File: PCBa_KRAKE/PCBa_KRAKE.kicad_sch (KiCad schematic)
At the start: 60 parts, among them J1 Conn_01x08, J101 Barrel_Jack_Switch_SMT, J102 0.100_2Pin, J103 0.100_2Pin, J105 S04B-XASK-1(LF)(SN)Rev2, U1 AMS1117-3.3, U101 LM7805_TO220, U102 PI_ATMEGA328P-AU-InOrder, U999 ESP32-WROOM-32D

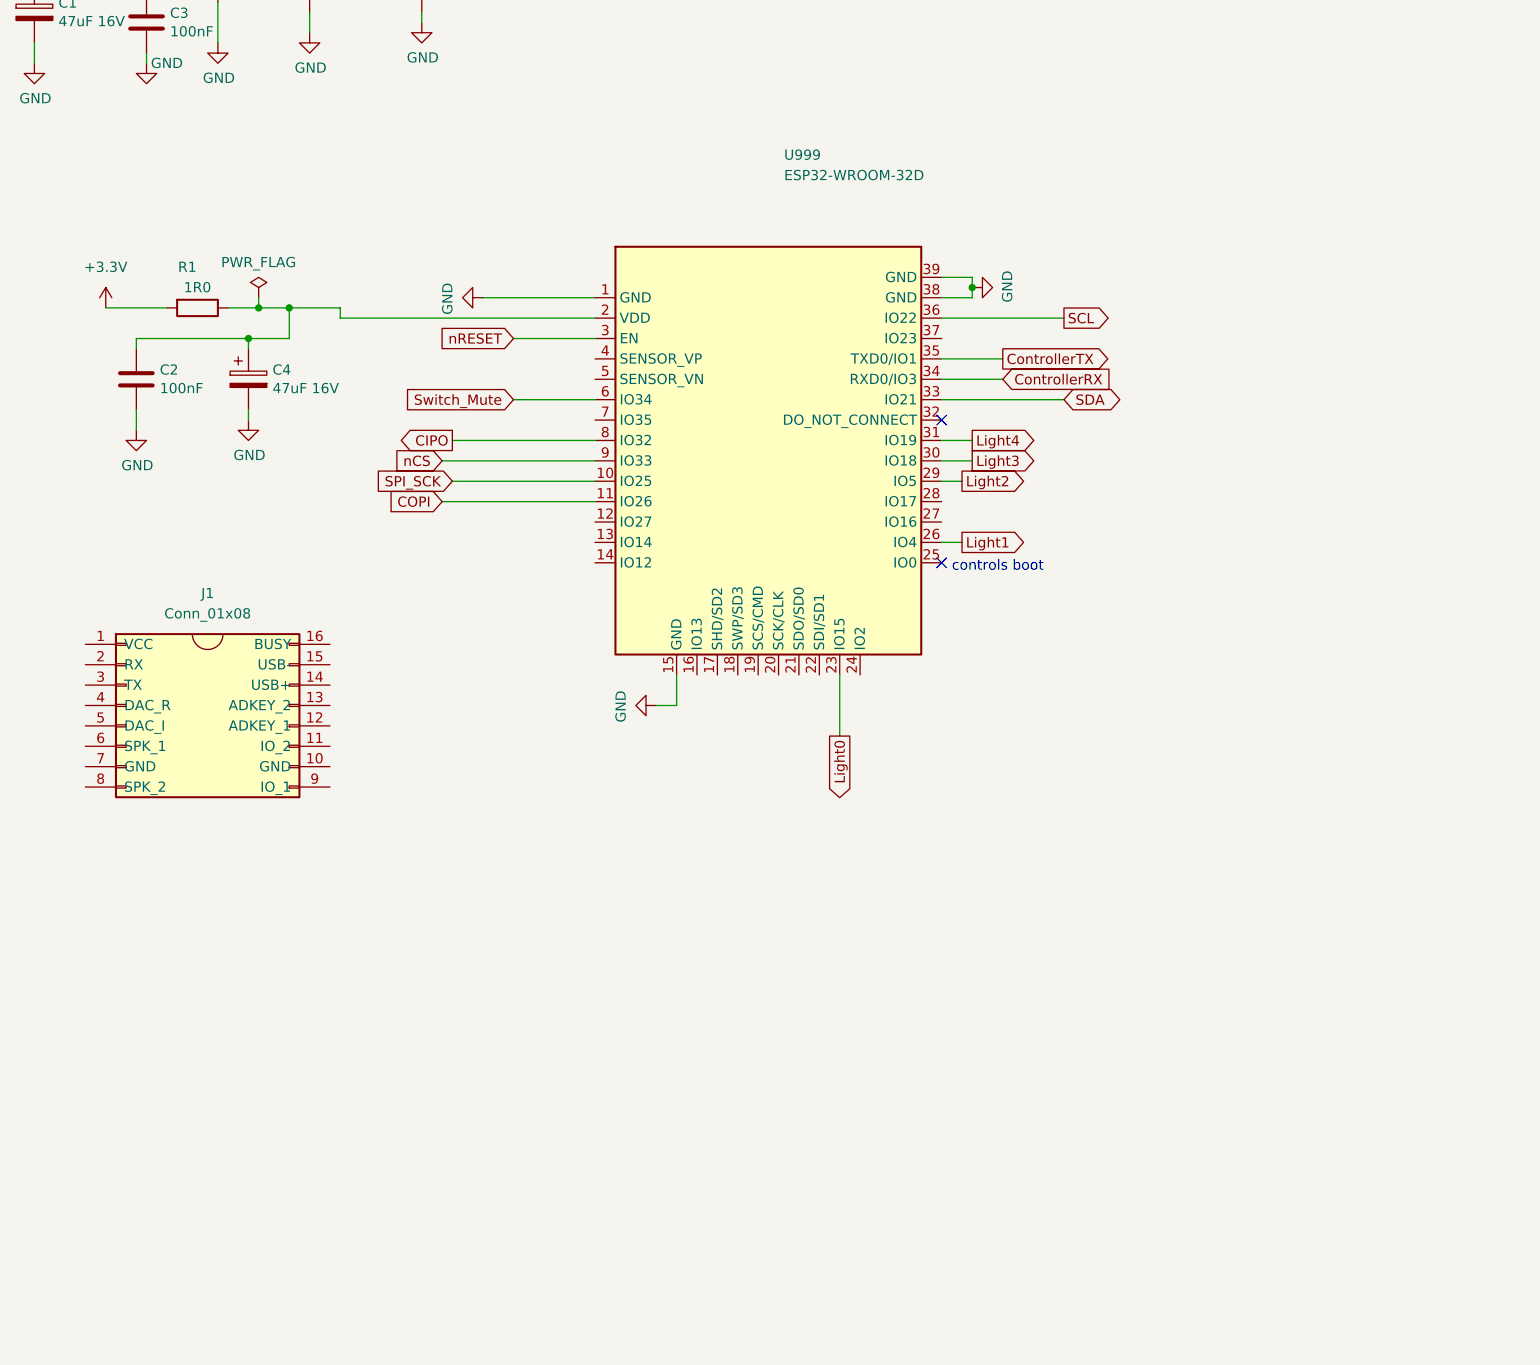
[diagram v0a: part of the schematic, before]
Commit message: Adding boot to load circuit, connected th DF player schematic symbol with the esp32, and editted the electric type of the module pins.
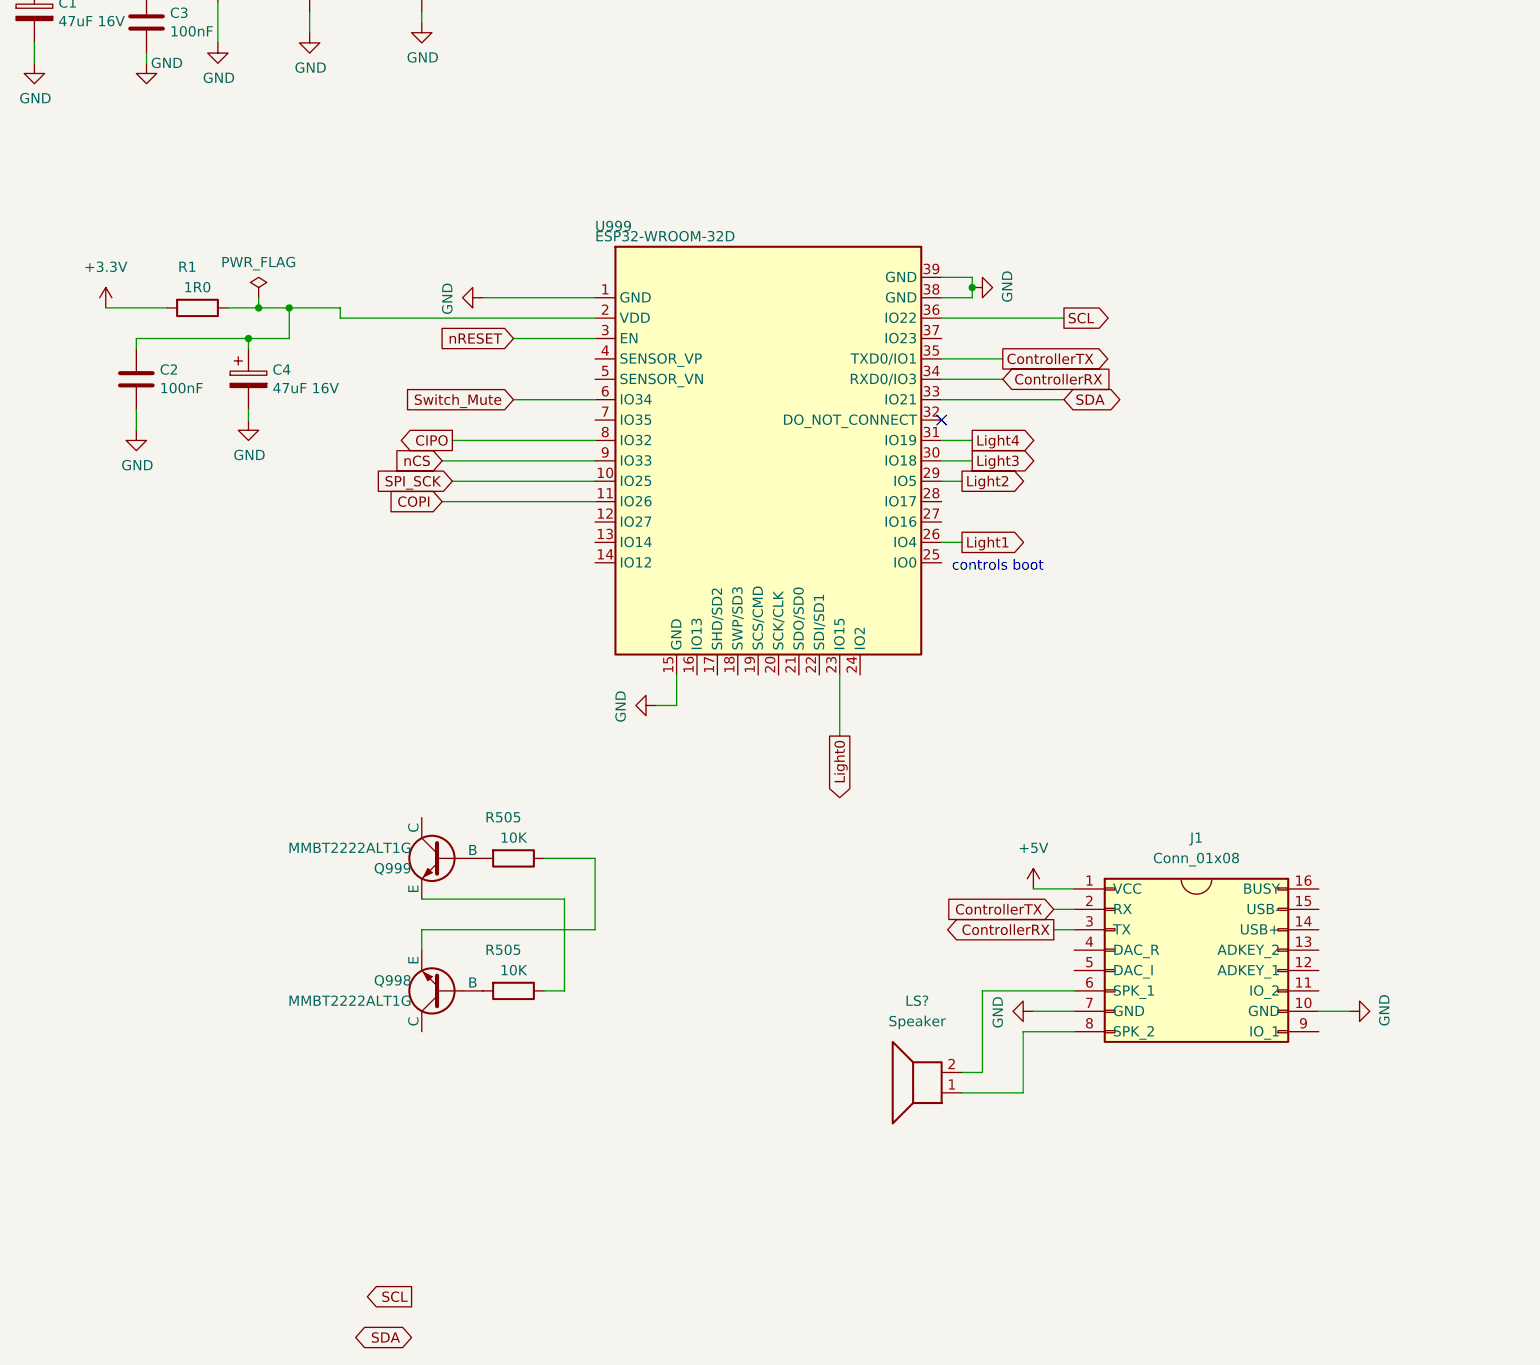
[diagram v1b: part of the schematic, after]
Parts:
- added LS?: Speaker, symbol Device:Speaker
- added Q998, Q999: MMBT2222ALT1G, symbol Simulation_SPICE:NPN
- added R505 (x2): 10K, Resistor_SMD:R_0603_1608Metric_Pad0.98x0.95mm_HandSolder, symbol Device:R
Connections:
- net +5V: now also J1.1 (VCC)
- net ControllerRX: now also J1.3 (TX)
- net ControllerTX: now also J1.2 (RX)
- net GND: now also J1.10 (GND), J1.7 (GND)
- net at J1.6 (SPK_1): now also LS?.2
- net at J1.8 (SPK_2): now also LS?.1
- new net: Q998.2 (B), R505.2
- new net: Q998.3 (E), R505.1
- new net: Q999.2 (B), R505.2
- new net: Q999.3 (E), R505.1
- no-connect marks 4 -> 3
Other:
- moved on the sheet: J1
